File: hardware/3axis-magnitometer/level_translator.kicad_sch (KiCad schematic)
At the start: 10 parts, among them Q1 BSS138, Q2 BSS138

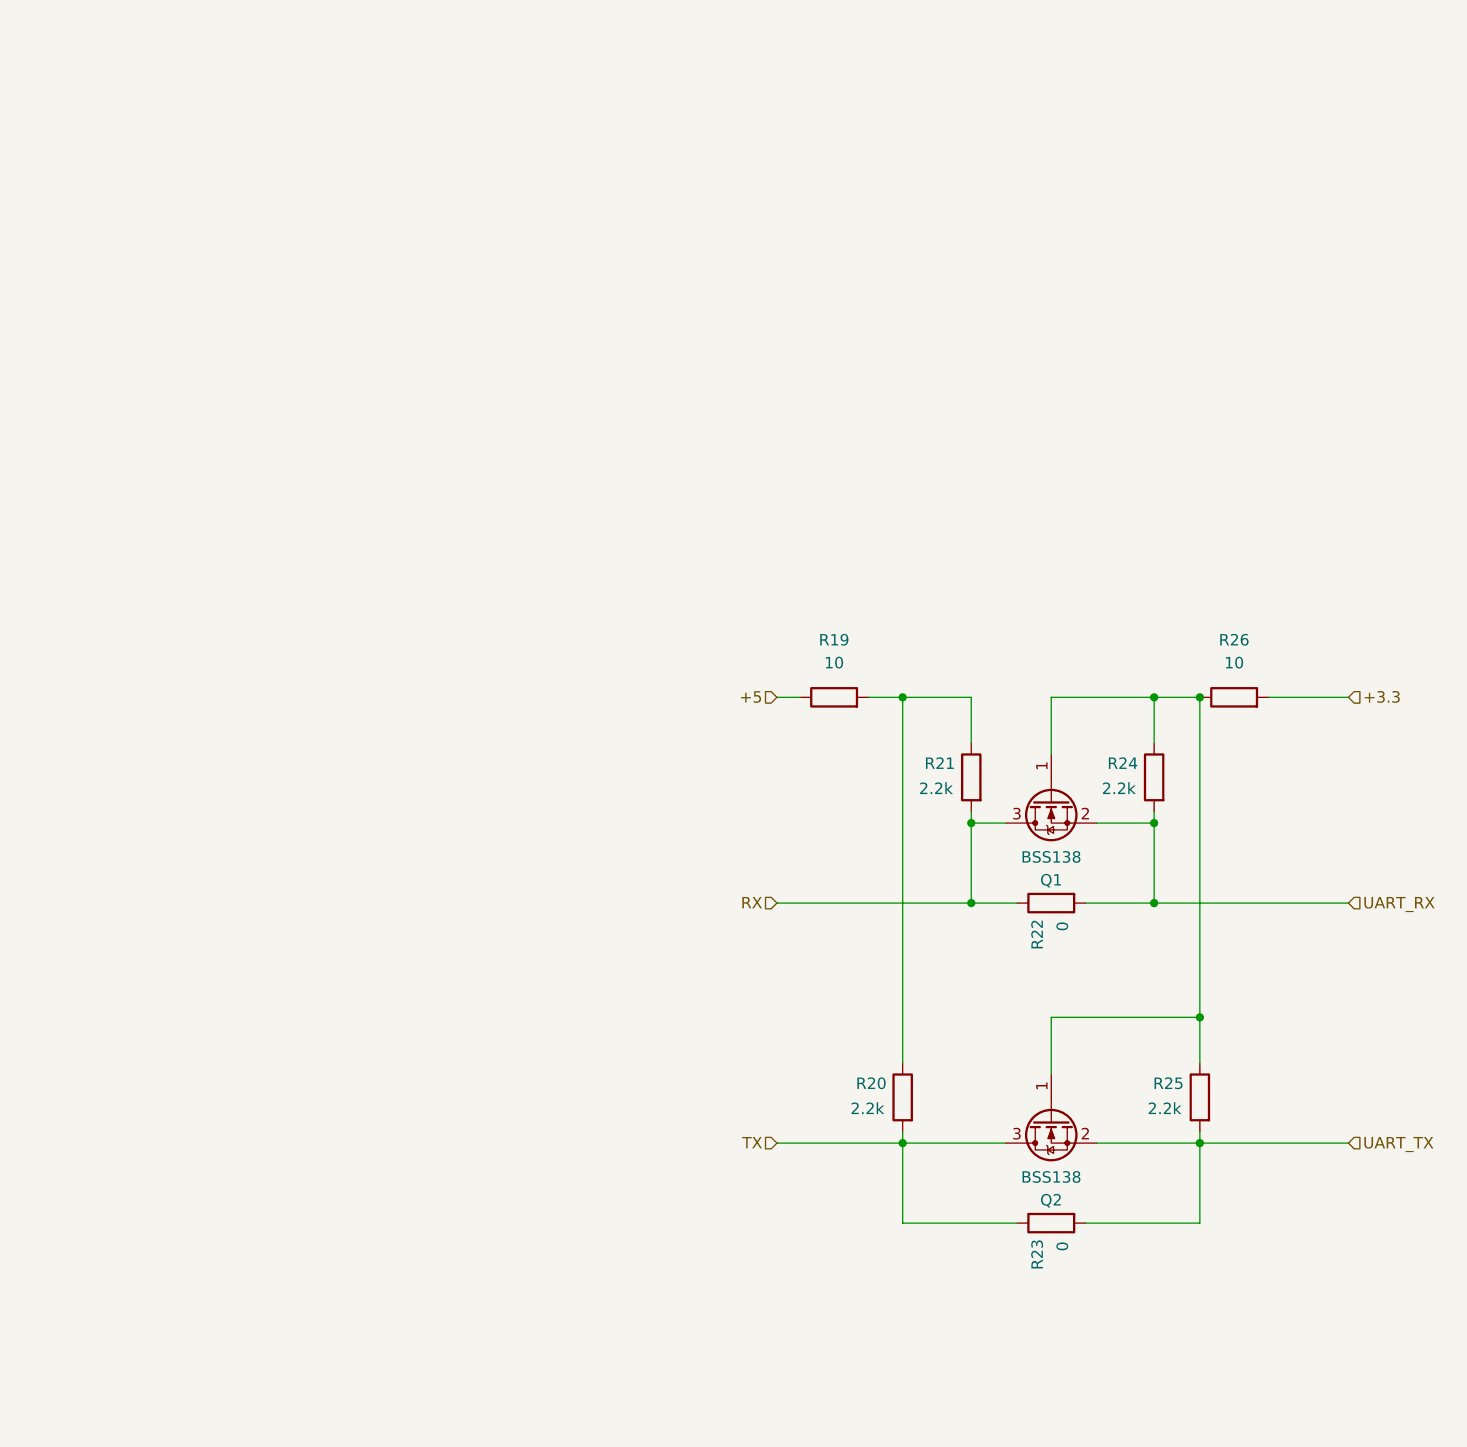
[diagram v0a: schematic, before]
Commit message: Add files via upload
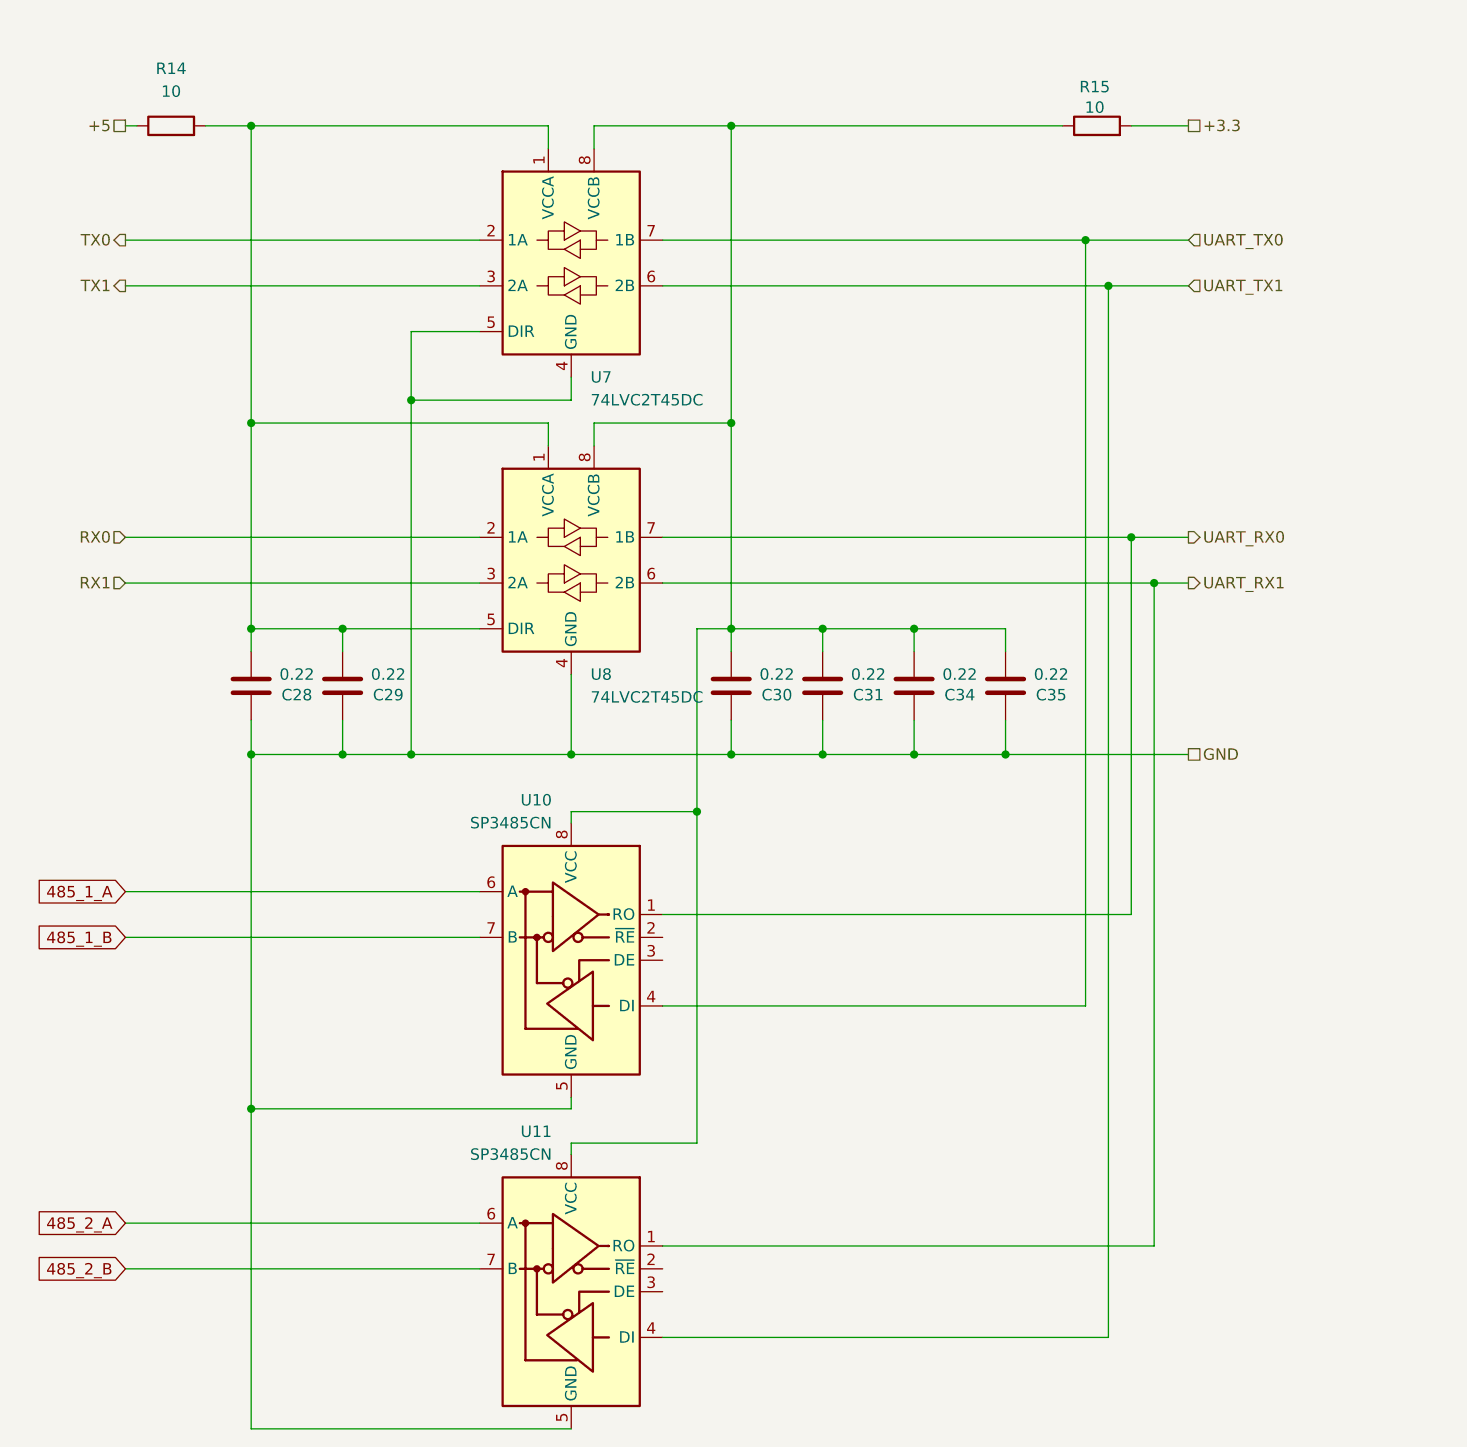
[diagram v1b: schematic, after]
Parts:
- removed Q1, Q2: BSS138, Package_TO_SOT_SMD:SOT-23, symbol Transistor_FET:BSS138
- removed R20, R21, R24, R25: 2.2k, Resistor_SMD:R_0805_2012Metric, symbol Device:R
- removed R22, R23: 0, Resistor_SMD:R_0805_2012Metric, symbol Device:R
- added C28, C29, C30, C31, C34, C35: 0.22, Capacitor_SMD:C_0805_2012Metric, symbol Device:C
- added U10, U11: SP3485CN, Package_SO:SOIC-8_3.9x4.9mm_P1.27mm, symbol Interface_UART:SP3485CN
- added U7, U8: 74LVC2T45DC, Package_SO:VSSOP-8_2.3x2mm_P0.5mm, symbol Logic_LevelTranslator:74LVC2T45DC
- renumbered R19 to R14, R26 to R15
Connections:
- net at R15.1: now also C30.1, C31.1, C34.1, C35.1, U10.8 (VCC), U11.8 (VCC), U7.8 (VCCB), U8.8 (VCCB)
- net at R14.2: now also C28.1, C29.1, U7.1 (VCCA), U8.1 (VCCA), U8.5 (DIR)
- new net 485_1_A: U10.6 (A)
- new net 485_1_B: U10.7 (B)
- new net 485_2_A: U11.6 (A)
- new net 485_2_B: U11.7 (B)
- new net GND: C28.2, C29.2, C30.2, C31.2, C34.2, C35.2, U10.5 (GND), U11.5 (GND), U7.4 (GND), U7.5 (DIR), U8.4 (GND)
- new net RX0: U8.2 (1A)
- new net RX1: U8.3 (2A)
- new net TX0: U7.2 (1A)
- new net TX1: U7.3 (2A)
- new net UART_RX0: U10.1 (RO), U8.7 (1B)
- new net UART_RX1: U11.1 (RO), U8.6 (2B)
- new net UART_TX0: U10.4 (DI), U7.7 (1B)
- new net UART_TX1: U11.4 (DI), U7.6 (2B)
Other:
- moved on the sheet: R14, R15

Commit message: начата новая трассировка
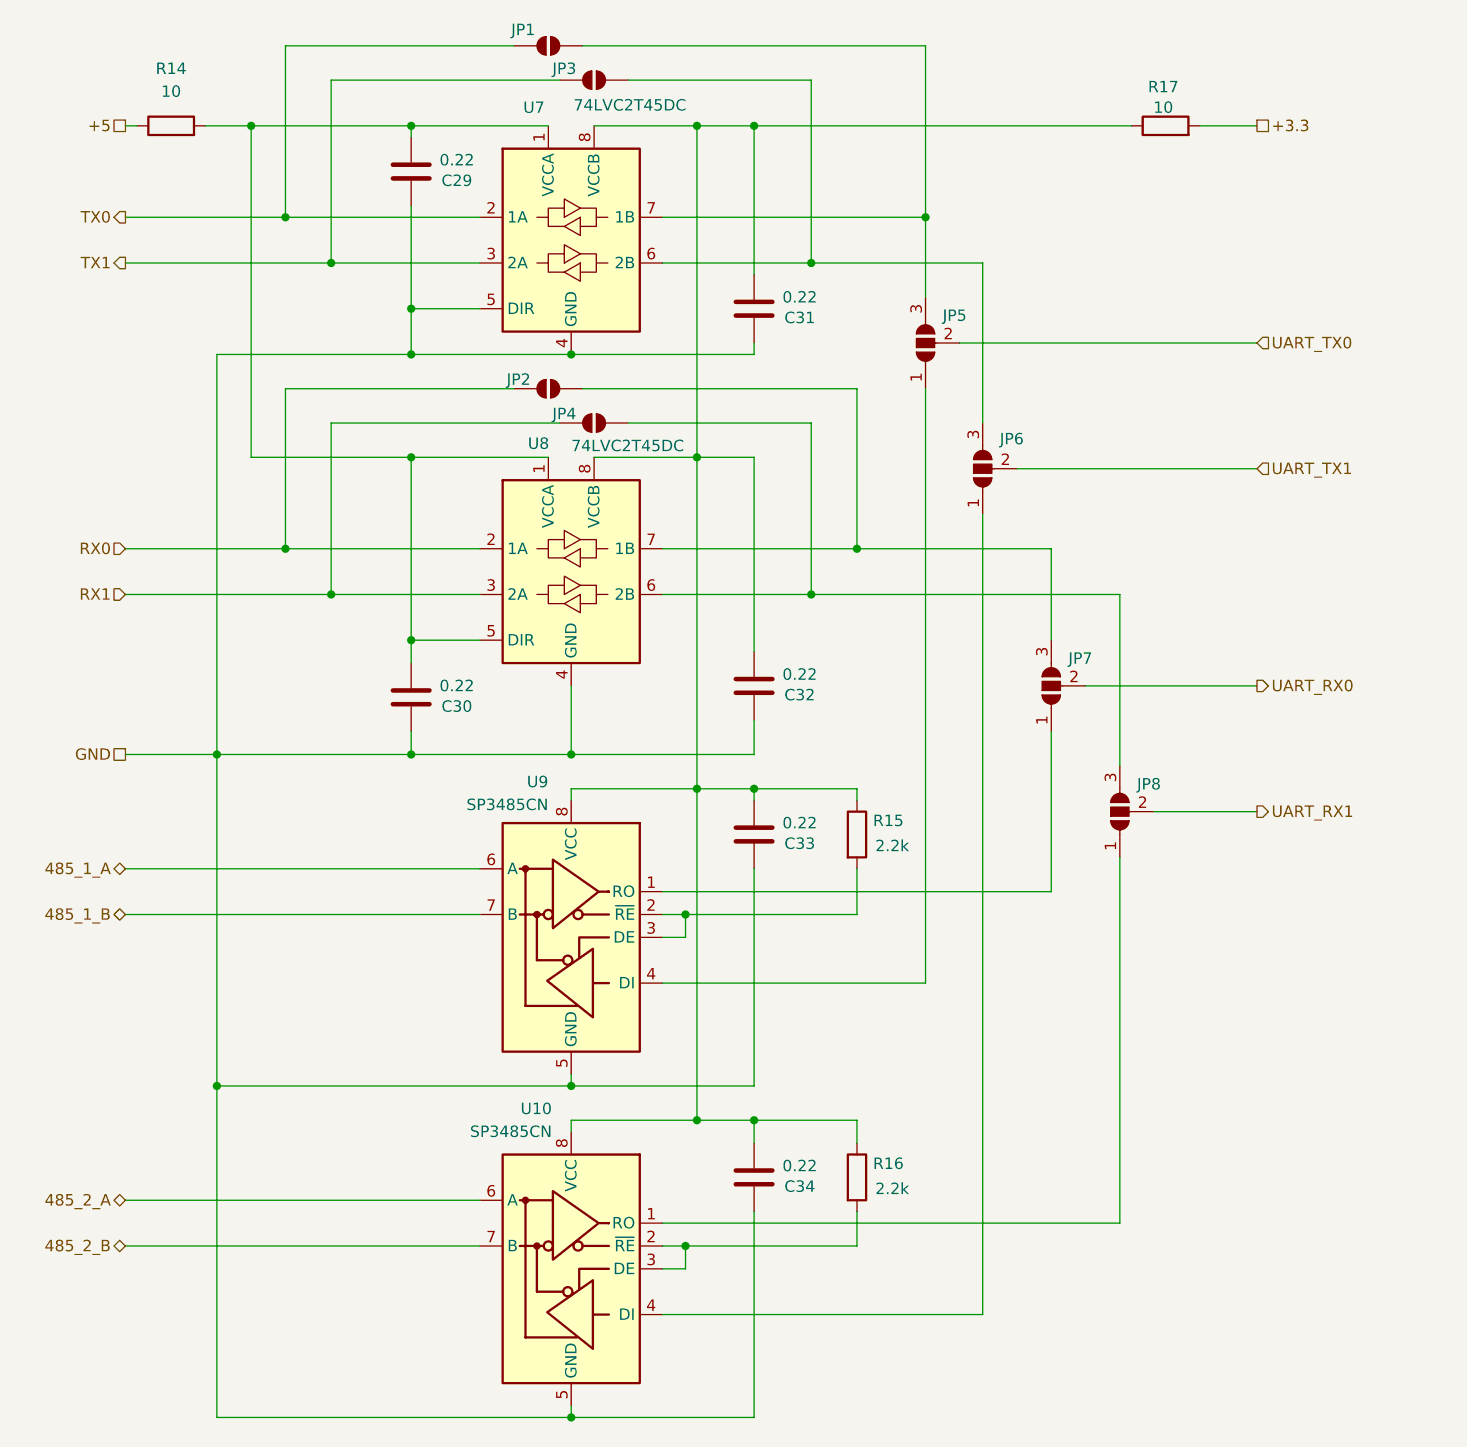
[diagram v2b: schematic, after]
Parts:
- added JP1, JP2, JP3, JP4: SolderJumper_2_Open, Jumper:SolderJumper-2_P1.3mm_Open_TrianglePad1.0x1.5mm, symbol Jumper:SolderJumper_2_Open
- added JP5, JP6, JP7, JP8: SolderJumper_3_Open, Jumper:SolderJumper-3_P2.0mm_Open_TrianglePad1.0x1.5mm_NumberLabels, symbol Jumper:SolderJumper_3_Open
- added R15, R16: 2.2k, Resistor_SMD:R_0805_2012Metric, symbol Device:R
- renumbered C28 to C29, C29 to C30, C30 to C32, C34 to C33, C35 to C34, R15 to R17, U11 to U10, U10 to U9
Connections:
- net RX0: now also JP2.1 (A)
- net RX1: now also JP4.1 (A)
- net TX0: now also JP1.1 (A)
- net TX1: now also JP3.1 (A)
- net UART_RX0: now also JP7.2 (C); no longer U8.7 (1B), U9.1 (RO)
- net UART_RX1: now also JP8.2 (C); no longer U10.1 (RO), U8.6 (2B)
- net UART_TX0: now also JP5.2 (C); no longer U7.7 (1B), U9.4 (DI)
- net UART_TX1: now also JP6.2 (C); no longer U10.4 (DI), U7.6 (2B)
- net at C31.1, C32.1, C33.1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: now also R15.1, R16.1
- net at U9.2 (~{RE}): now also U9.3 (DE), R15.2
- net at U10.2 (~{RE}): now also U10.3 (DE), R16.2
- new net: JP3.2 (B), JP6.3 (B), U7.6 (2B)
- new net: JP1.2 (B), JP5.3 (B), U7.7 (1B)
- new net: JP6.1 (A), U10.4 (DI)
- new net: JP7.1 (A), U9.1 (RO)
- new net: JP2.2 (B), JP7.3 (B), U8.7 (1B)
- new net: JP4.2 (B), JP8.3 (B), U8.6 (2B)
- new net: JP5.1 (A), U9.4 (DI)
- new net: JP8.1 (A), U10.1 (RO)
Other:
- moved on the sheet: C29, C30, C31, C32, C33, C34, R17, U10, U7, U8, U9

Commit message: трасировка магнитометра
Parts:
- JP1, JP2, JP3, JP4: footprint Jumper:SolderJumper-2_P1.3mm_Open_TrianglePad1.0x1.5mm -> Jumper:SolderJumper-2_P1.3mm_Open_Pad1.0x1.5mm
- JP5, JP6, JP7, JP8: footprint Jumper:SolderJumper-3_P2.0mm_Open_TrianglePad1.0x1.5mm_NumberLabels -> Jumper:SolderJumper-3_P1.3mm_Open_Pad1.0x1.5mm
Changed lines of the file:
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@@
 			)
 		)
-		(property "Footprint" "Jumper:SolderJumper-3_P2.0mm_Open_TrianglePad1.0x1.5mm_NumberLabels"
+		(property "Footprint" "Jumper:SolderJumper-3_P1.3mm_Open_Pad1.0x1.5mm"
 			(at 137.16 68.58 0)
 			(effects
@@
 			)
 		)
-		(property "Footprint" "Jumper:SolderJumper-3_P2.0mm_Open_TrianglePad1.0x1.5mm_NumberLabels"
+		(property "Footprint" "Jumper:SolderJumper-3_P1.3mm_Open_Pad1.0x1.5mm"
 			(at 144.78 92.71 0)
 			(effects
@@
 			)
 		)
-		(property "Footprint" "Jumper:SolderJumper-2_P1.3mm_Open_TrianglePad1.0x1.5mm"
+		(property "Footprint" "Jumper:SolderJumper-2_P1.3mm_Open_Pad1.0x1.5mm"
 			(at 93.98 25.4 0)
 			(effects
@@
 			)
 		)
-		(property "Footprint" "Jumper:SolderJumper-2_P1.3mm_Open_TrianglePad1.0x1.5mm"
+		(property "Footprint" "Jumper:SolderJumper-2_P1.3mm_Open_Pad1.0x1.5mm"
 			(at 93.98 63.5 0)
 			(effects
@@
 			)
 		)
-		(property "Footprint" "Jumper:SolderJumper-2_P1.3mm_Open_TrianglePad1.0x1.5mm"
+		(property "Footprint" "Jumper:SolderJumper-2_P1.3mm_Open_Pad1.0x1.5mm"
 			(at 88.9 59.69 0)
 			(effects
@@
 			)
 		)
-		(property "Footprint" "Jumper:SolderJumper-2_P1.3mm_Open_TrianglePad1.0x1.5mm"
+		(property "Footprint" "Jumper:SolderJumper-2_P1.3mm_Open_Pad1.0x1.5mm"
 			(at 88.9 21.59 0)
 			(effects
@@
 			)
 		)
-		(property "Footprint" "Jumper:SolderJumper-3_P2.0mm_Open_TrianglePad1.0x1.5mm_NumberLabels"
+		(property "Footprint" "Jumper:SolderJumper-3_P1.3mm_Open_Pad1.0x1.5mm"
 			(at 130.81 54.61 0)
 			(effects
@@
 			)
 		)
-		(property "Footprint" "Jumper:SolderJumper-3_P2.0mm_Open_TrianglePad1.0x1.5mm_NumberLabels"
+		(property "Footprint" "Jumper:SolderJumper-3_P1.3mm_Open_Pad1.0x1.5mm"
 			(at 152.4 106.68 0)
 			(effects
